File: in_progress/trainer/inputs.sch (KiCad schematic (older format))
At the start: 45 parts

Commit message: .
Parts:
- C? (x5): symbol C -> C-RESCUE-trainer
- R? (x5): symbol R -> R-RESCUE-trainer
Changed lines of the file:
@@
 LIBS:memory
 LIBS:xilinx
-LIBS:special
 LIBS:microcontrollers
 LIBS:dsp
@@
 LIBS:valves
 LIBS:MiscellaneousDevices
+LIBS:ULN280xA
 LIBS:Gajda_cmosieee
 LIBS:jhd-162a
 LIBS:capteurs
 LIBS:trainer-cache
-EELAYER 27 0
+EELAYER 25 0
 EELAYER END
 $Descr A4 11693 8268
@@
 $EndComp
 $Comp
-L R R?
+L R-RESCUE-trainer R?
 U 1 1 56563A1D
 P 7600 3950
@@
 $EndComp
 $Comp
-L C C?
+L C-RESCUE-trainer C?
 U 1 1 56563A2B
 P 7600 4250
+AR Path="/56563A2B" Ref="C?"  Part="1"
+AR Path="/5655FD48/56563A2B" Ref="C?"  Part="1"
 F 0 "C?" H 7625 4350 50  0000 L CNN
 F 1 "C" H 7625 4150 50  0000 L CNN
@@
 $EndComp
 $Comp
-L R R?
+L R-RESCUE-trainer R?
 U 1 1 56563A40
 P 7600 5000
@@
 $EndComp
 $Comp
-L C C?
+L C-RESCUE-trainer C?
 U 1 1 56563A4E
 P 7600 5300
+AR Path="/56563A4E" Ref="C?"  Part="1"
+AR Path="/5655FD48/56563A4E" Ref="C?"  Part="1"
 F 0 "C?" H 7625 5400 50  0000 L CNN
 F 1 "C" H 7625 5200 50  0000 L CNN
@@
 $EndComp
 $Comp
-L R R?
+L R-RESCUE-trainer R?
 U 1 1 56563A63
 P 10200 3950
@@
 $EndComp
 $Comp
-L C C?
+L C-RESCUE-trainer C?
 U 1 1 56563A71
 P 10200 4250
+AR Path="/56563A71" Ref="C?"  Part="1"
+AR Path="/5655FD48/56563A71" Ref="C?"  Part="1"
 F 0 "C?" H 10225 4350 50  0000 L CNN
 F 1 "C" H 10225 4150 50  0000 L CNN
@@
 $EndComp
 $Comp
-L R R?
+L R-RESCUE-trainer R?
 U 1 1 56563A86
 P 10200 5000
@@
 $EndComp
 $Comp
-L C C?
+L C-RESCUE-trainer C?
 U 1 1 56563A94
 P 10200 5300
+AR Path="/56563A94" Ref="C?"  Part="1"
+AR Path="/5655FD48/56563A94" Ref="C?"  Part="1"
 F 0 "C?" H 10225 5400 50  0000 L CNN
 F 1 "C" H 10225 5200 50  0000 L CNN
@@
 $EndComp
 $Comp
-L R R?
+L R-RESCUE-trainer R?
 U 1 1 5657334B
 P 5350 4900
@@
 $EndComp
 $Comp
-L C C?
+L C-RESCUE-trainer C?
 U 1 1 56573357
 P 5350 5200
+AR Path="/56573357" Ref="C?"  Part="1"
+AR Path="/5655FD48/56573357" Ref="C?"  Part="1"
 F 0 "C?" H 5375 5300 50  0000 L CNN
 F 1 "C" H 5375 5100 50  0000 L CNN

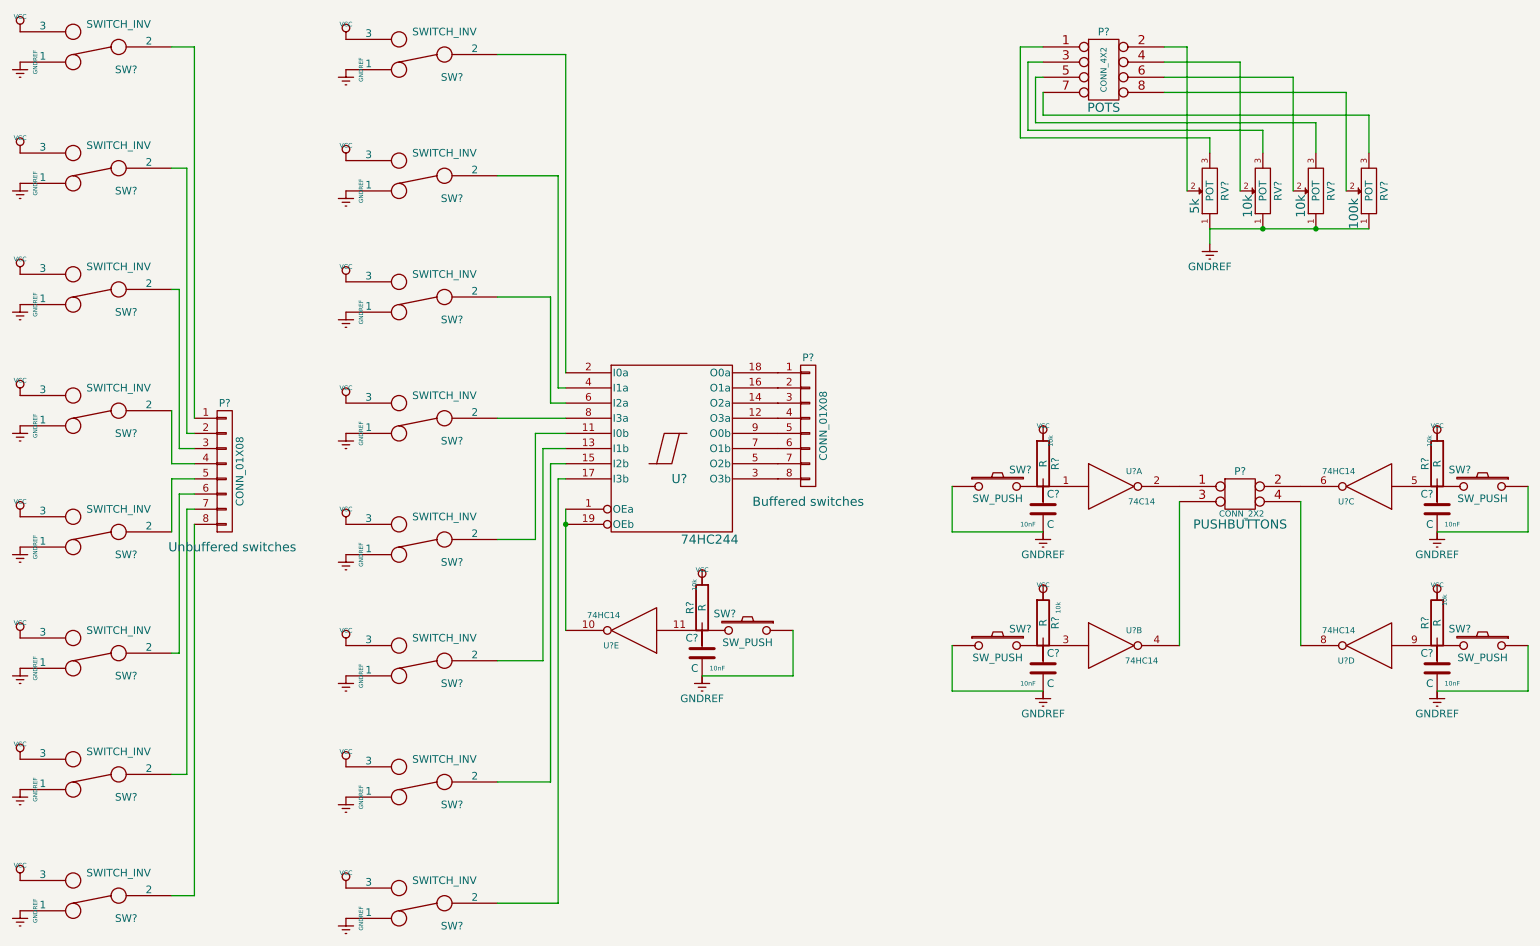
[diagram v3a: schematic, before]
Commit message: .
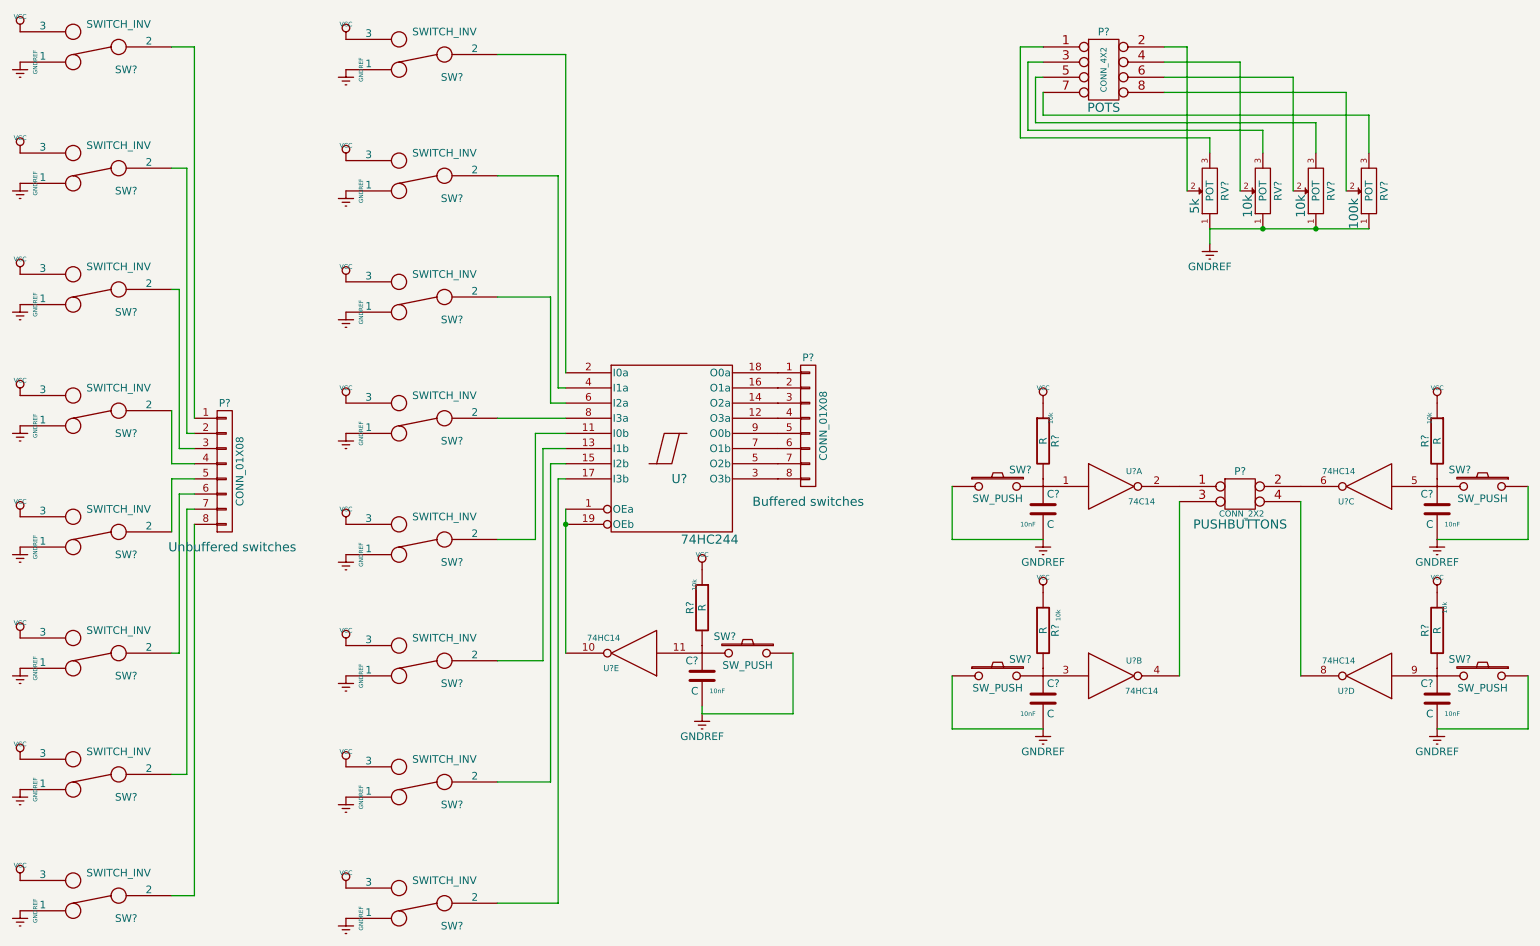
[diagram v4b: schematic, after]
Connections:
- net GNDREF: now also C?.2, C?.2, C?.2, C?.2, C?.2
- net VCC: now also R?.1, R?.1, R?.1, R?.1, R?.1
- net at R?.2: now also C?.1 (x5)
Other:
- moved on the sheet: C?, R?, SW?, U?B, U?D, U?E

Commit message: .
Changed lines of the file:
@@
 	8550 1200 8550 2150
 Wire Wire Line
-	8700 2400 9050 2400
-Wire Wire Line
-	9050 2400 9400 2400
-Wire Wire Line
-	9400 2400 9750 2400
+	8700 2400 9750 2400
 Connection ~ 9050 2400
 Connection ~ 9400 2400
@@
 $EndComp
 Wire Wire Line
-	4450 4250 4450 4350
-Wire Wire Line
-	4450 4350 4450 5200
+	4450 4250 4450 5200
 Connection ~ 4450 4350
 Wire Wire Line
